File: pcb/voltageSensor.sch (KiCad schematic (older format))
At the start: 3 parts

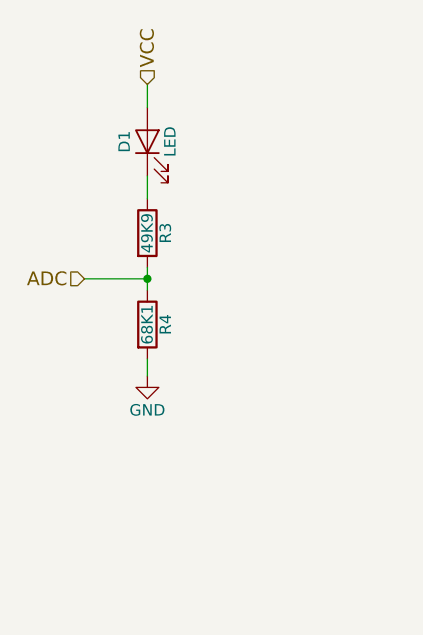
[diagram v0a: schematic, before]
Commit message: Clean up Kicad and TCC
Some changes in the
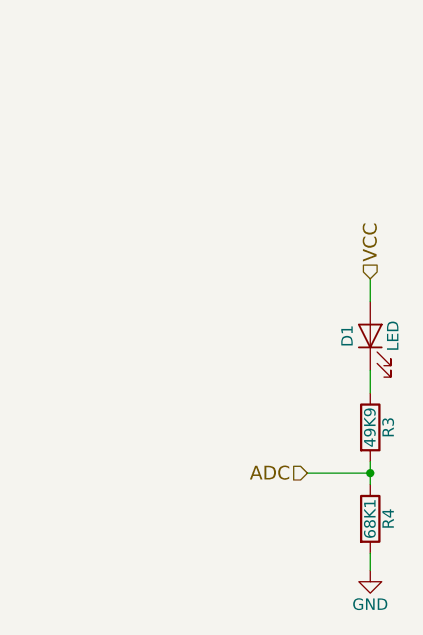
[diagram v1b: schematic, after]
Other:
- moved on the sheet: D1, R3, R4
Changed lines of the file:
@@
 $Descr A4 11693 8268
 encoding utf-8
-Sheet 9 10
-Title ""
+Sheet 8 10
+Title "Voltage Sensor Schematic"
 Date ""
-Rev ""
-Comp ""
+Rev "1"
+Comp "Universidade de Brasília - Campus Gama"
 Comment1 ""
 Comment2 ""
@@
 L Device:R R3
 U 1 1 5CD444E3
-P 5250 2750
-F 0 "R3" V 5330 2750 50  0000 C CNN
-F 1 "49K9" V 5250 2750 50  0000 C CNN
-F 2 "Resistors_SMD:R_1206" V 5180 2750 50  0001 C CNN
-F 3 "https://www.digikey.com/product-detail/en/panasonic-electronic-components/ERA-8AEB4992V/P49.9KBCCT-ND/3069837" H 5250 2750 50  0001 C CNN
-	1    5250 2750
+P 6225 3600
+F 0 "R3" V 6305 3600 50  0000 C CNN
+F 1 "49K9" V 6225 3600 50  0000 C CNN
+F 2 "Resistors_SMD:R_1206" V 6155 3600 50  0001 C CNN
+F 3 "https://www.digikey.com/product-detail/en/panasonic-electronic-components/ERA-8AEB4992V/P49.9KBCCT-ND/3069837" H 6225 3600 50  0001 C CNN
+	1    6225 3600
 	1    0    0    -1
 $EndComp
@@
 L Device:R R4
 U 1 1 5CD444FA
-P 5250 3150
-F 0 "R4" V 5330 3150 50  0000 C CNN
-F 1 "68K1" V 5250 3150 50  0000 C CNN
-F 2 "Resistors_SMD:R_1206" V 5180 3150 50  0001 C CNN
-F 3 "https://www.digikey.com/product-detail/en/stackpole-electronics-inc/RNCP1206FTD68K1/RNCP1206FTD68K1CT-ND/2240736" H 5250 3150 50  0001 C CNN
-	1    5250 3150
+P 6225 4000
+F 0 "R4" V 6305 4000 50  0000 C CNN
+F 1 "68K1" V 6225 4000 50  0000 C CNN
+F 2 "Resistors_SMD:R_1206" V 6155 4000 50  0001 C CNN
+F 3 "https://www.digikey.com/product-detail/en/stackpole-electronics-inc/RNCP1206FTD68K1/RNCP1206FTD68K1CT-ND/2240736" H 6225 4000 50  0001 C CNN
+	1    6225 4000
 	1    0    0    -1
 $EndComp
@@
 L Device:LED D1
 U 1 1 5CD44513
-P 5250 2350
-F 0 "D1" H 5250 2450 50  0000 C CNN
-F 1 "LED" H 5250 2250 50  0000 C CNN
-F 2 "Resistors_SMD:R_0603" H 5250 2350 50  0001 C CNN
-F 3 "https://www.digikey.com/product-detail/en/rohm-semiconductor/SML-D12U1WT86/SML-D12U1WT86CT-ND/5843858" H 5250 2350 50  0001 C CNN
-	1    5250 2350
+P 6225 3200
+F 0 "D1" H 6225 3300 50  0000 C CNN
+F 1 "LED" H 6225 3100 50  0000 C CNN
+F 2 "Resistors_SMD:R_0603" H 6225 3200 50  0001 C CNN
+F 3 "https://www.digikey.com/product-detail/en/rohm-semiconductor/SML-D12U1WT86/SML-D12U1WT86CT-ND/5843858" H 6225 3200 50  0001 C CNN
+	1    6225 3200
 	0    -1   -1   0
 $EndComp
-Text HLabel 5250 2100 1    60   Input ~ 0
+Text HLabel 6225 2950 1    60   Input ~ 0
 VCC
 Wire Wire Line
-	5250 2100 5250 2200
+	6225 2950 6225 3050
 Wire Wire Line
-	5250 2500 5250 2600
+	6225 3350 6225 3450
 Wire Wire Line
-	5250 2900 5250 2950
+	6225 3750 6225 3800
 $Comp
 L power:GND #PWR017
 U 1 1 5CD4858F
-P 5250 3375
-F 0 "#PWR017" H 5250 3125 50  0001 C CNN
-F 1 "GND" H 5250 3225 50  0000 C CNN
-F 2 "" H 5250 3375 50  0001 C CNN
-F 3 "" H 5250 3375 50  0001 C CNN
-	1    5250 3375
+P 6225 4225
+F 0 "#PWR017" H 6225 3975 50  0001 C CNN
+F 1 "GND" H 6225 4075 50  0000 C CNN
+F 2 "" H 6225 4225 50  0001 C CNN
+F 3 "" H 6225 4225 50  0001 C CNN
+	1    6225 4225
 	1    0    0    -1
 $EndComp
-Text HLabel 4975 2950 0    60   Input ~ 0
+Text HLabel 5950 3800 0    60   Input ~ 0
 ADC
 Wire Wire Line
-	4975 2950 5250 2950
-Connection ~ 5250 2950
+	5950 3800 6225 3800
+Connection ~ 6225 3800
 Wire Wire Line
-	5250 3300 5250 3375
+	6225 4150 6225 4225
 Wire Wire Line
-	5250 2950 5250 3000
+	6225 3800 6225 3850
 $EndSCHEMATC
